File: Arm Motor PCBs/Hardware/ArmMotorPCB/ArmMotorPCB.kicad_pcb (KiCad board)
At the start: 2 copper layers, 21.6 x 27.9 mm, 3 parts

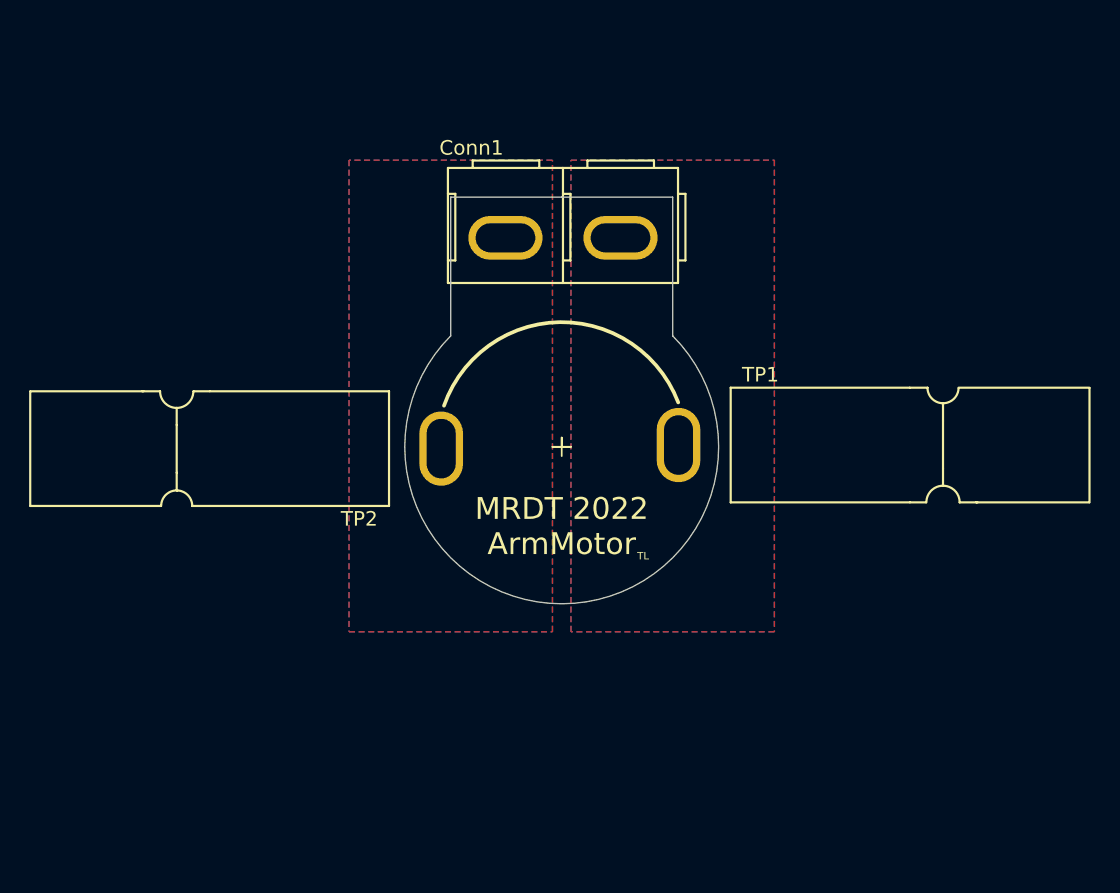
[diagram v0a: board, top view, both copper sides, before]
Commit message: gerbs added and zipped
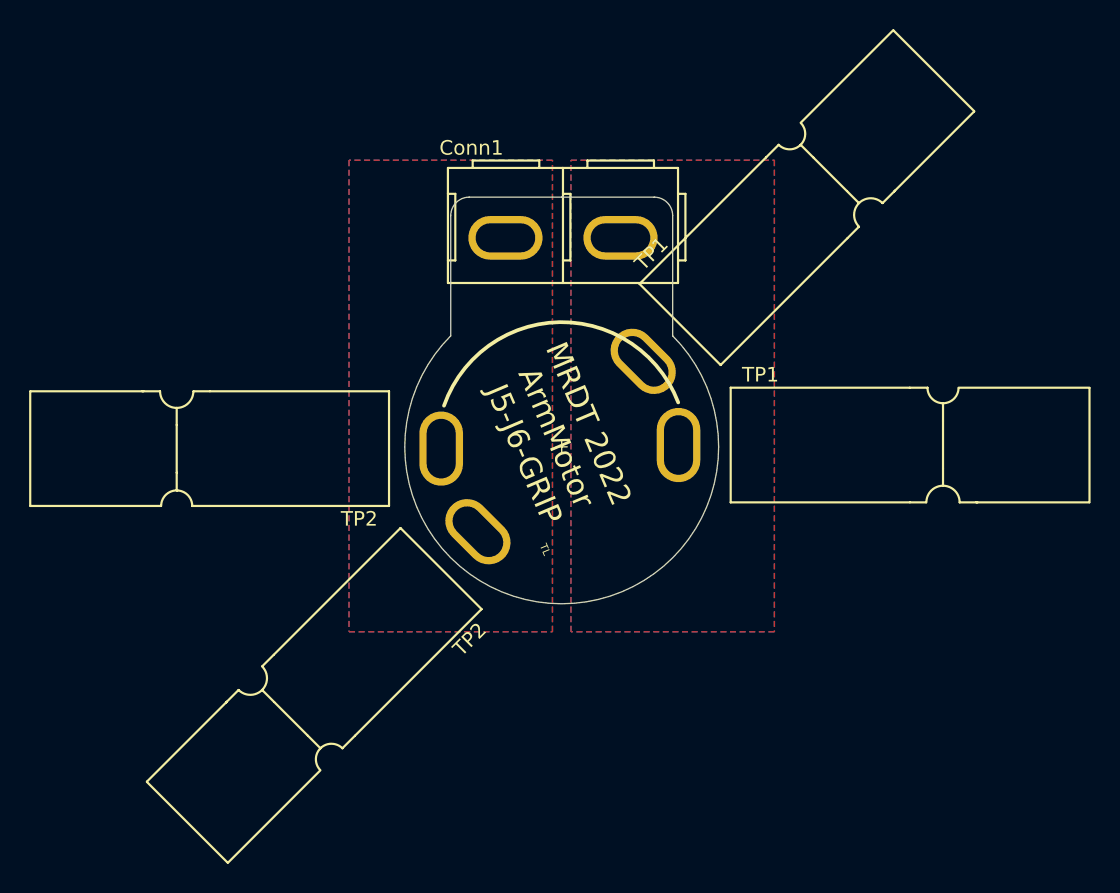
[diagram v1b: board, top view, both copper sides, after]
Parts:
- added TP1: TestPoint, MRDT_Connectors:Square_Anderson_1_H, F.Cu at (143.3, 57.9)
- added TP2: TestPoint, MRDT_Connectors:Square_Anderson_1_H, F.Cu at (132.1, 69.0)
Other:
- outline, holes or cut-outs redrawn
- board text added: "J5-J6-GRIP"
